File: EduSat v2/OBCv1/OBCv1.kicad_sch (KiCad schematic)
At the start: 10 parts, among them J1 Conn_02x20_Odd_Even, J2 USB_C_Receptacle_USB2.0_16P, U1 ESP32-WROOM-32E, U2 CP2102N-Axx-xQFN28, U3 Ai-Thinker-Ra-02

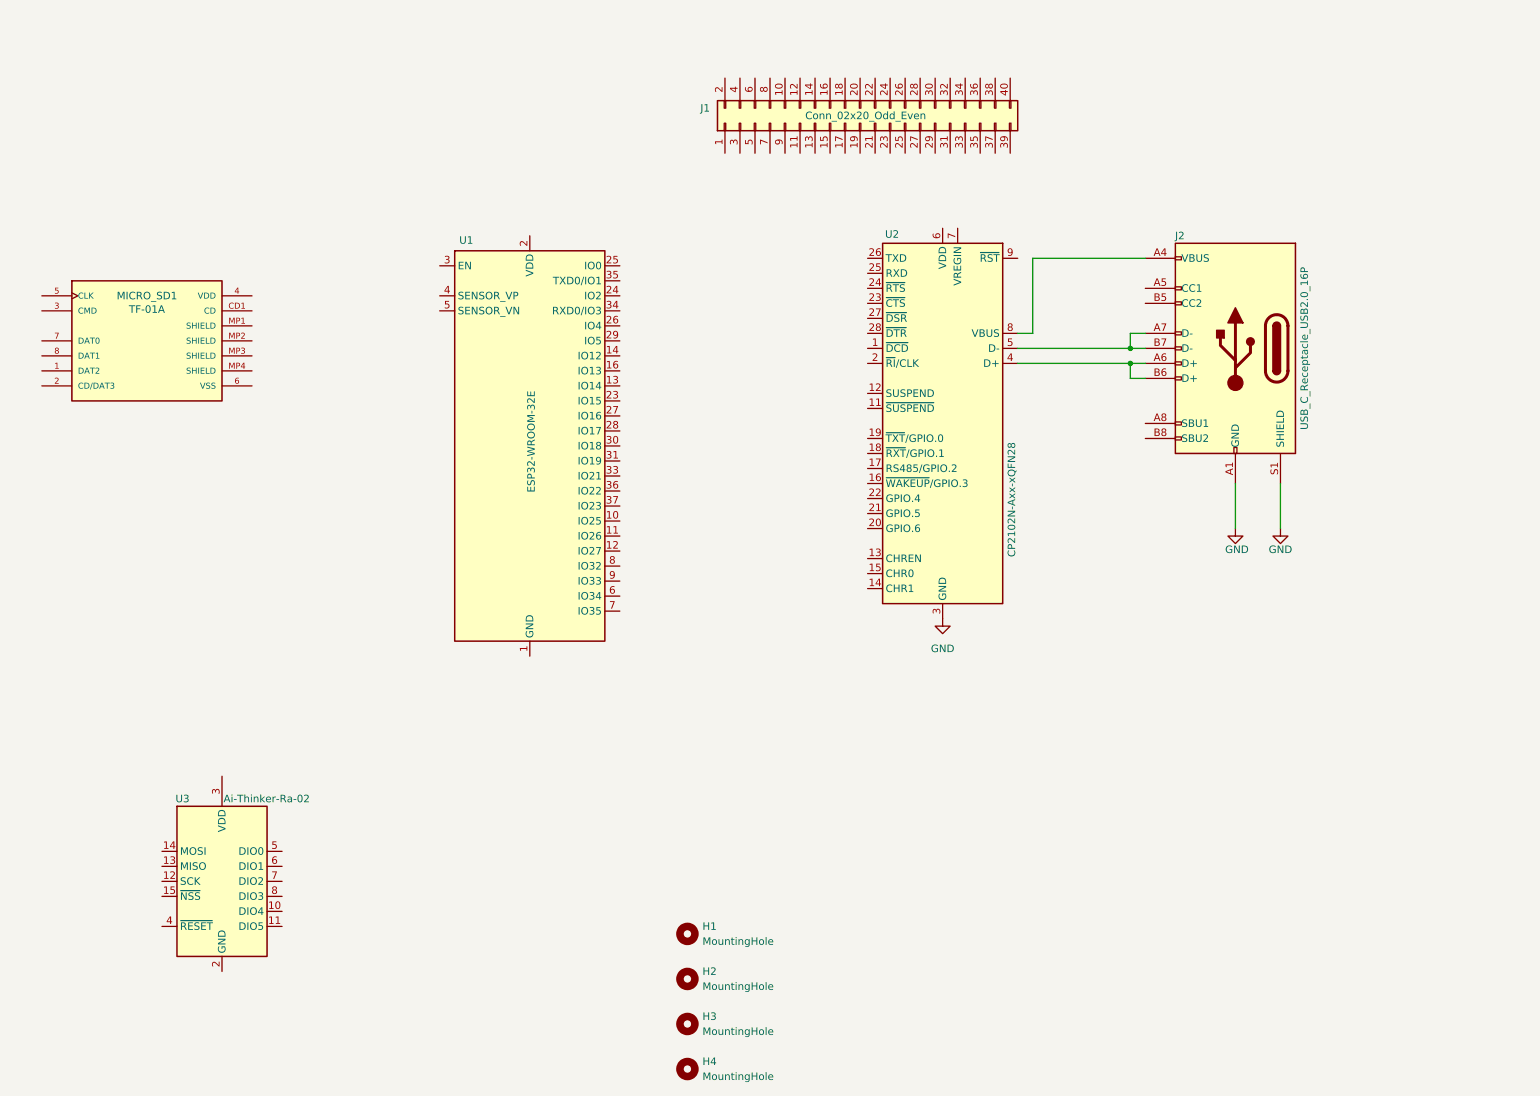
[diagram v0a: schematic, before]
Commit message: a
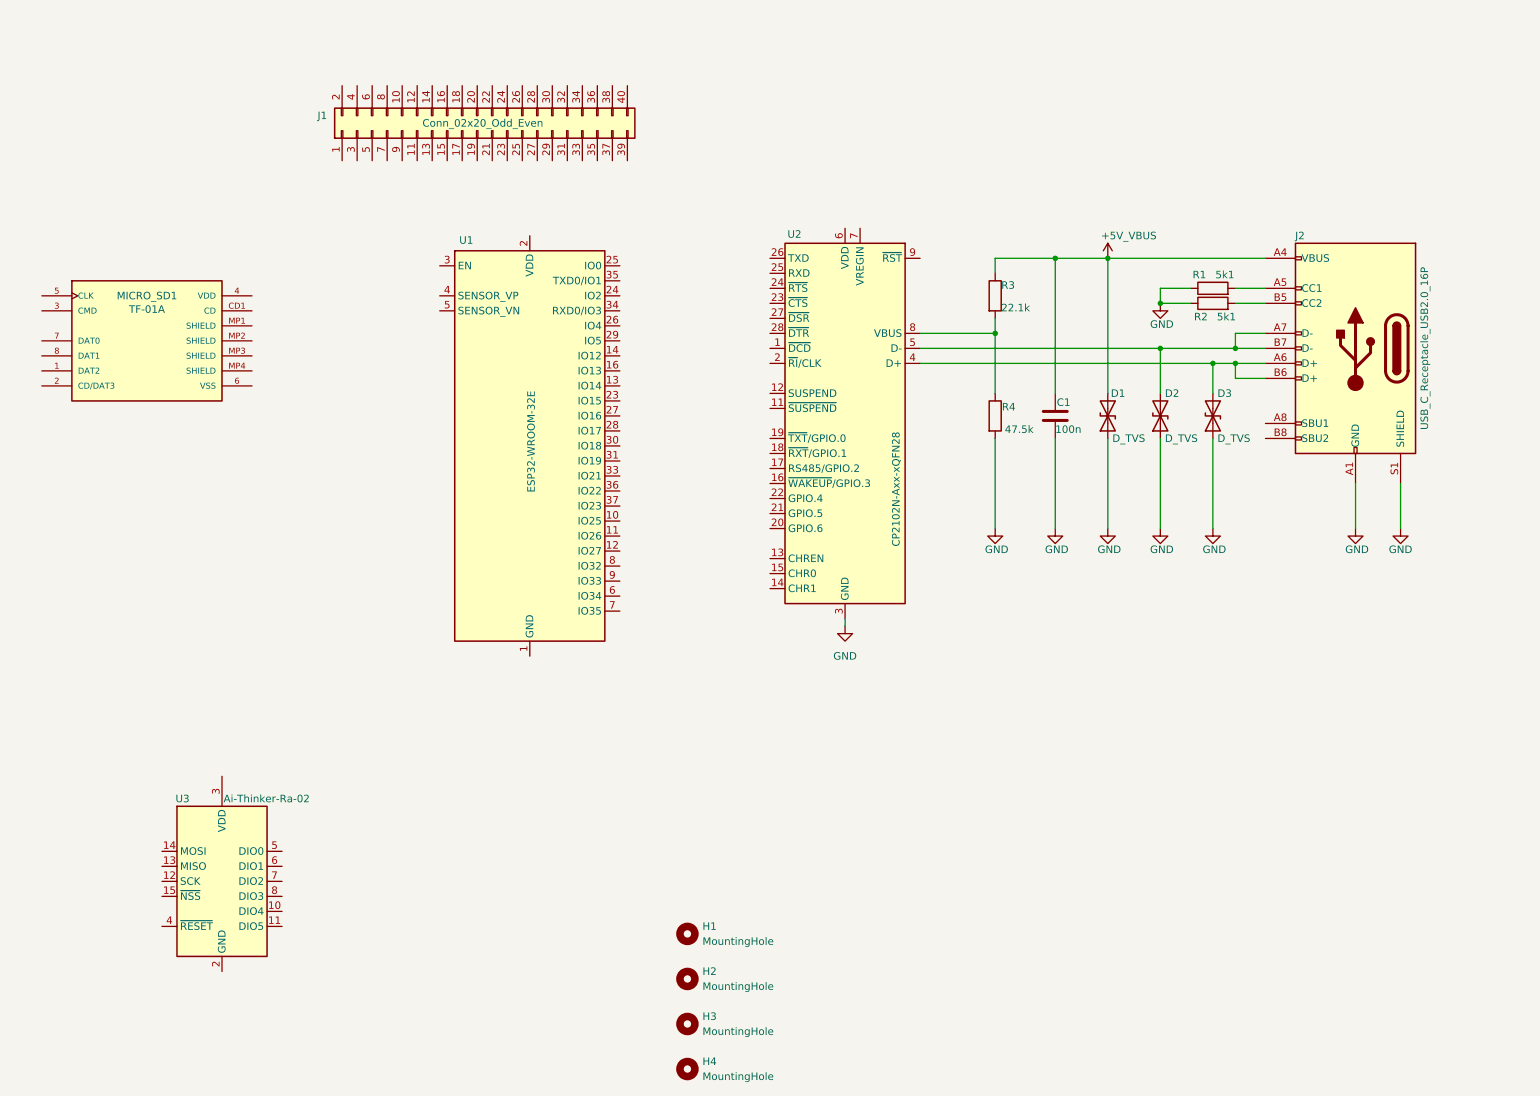
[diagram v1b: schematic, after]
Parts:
- added C1: 100n, Capacitor_SMD:C_0805_2012Metric, symbol Device:C
- added D1, D2, D3: D_TVS, Diode_SMD:D_0603_1608Metric, symbol Device:D_TVS
- added R1, R2: 5k1, Resistor_SMD:R_0805_2012Metric, symbol Device:R
- added R3: 22.1k, symbol Device:R
- added R4: 47.5k, symbol Device:R
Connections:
- net GND: now also C1.2, D1.1 (A1), D2.1 (A1), D3.1 (A1), R1.1, R2.1, R4.2
- net +5V_VBUS: now reaches J2.A4 (VBUS), J2.A9 (VBUS), J2.B4 (VBUS), J2.B9 (VBUS)
- net +5V_VBUS: now also C1.1, D1.2 (A2), R3.1; no longer U2.8 (VBUS)
- net at J2.A5 (CC1): now also R1.2
- net at J2.A6 (D+), J2.B6 (D+), U2.4 (D+): now also D3.2 (A2)
- net at J2.A7 (D-), J2.B7 (D-), U2.5 (D-): now also D2.2 (A2)
- net at J2.B5 (CC2): now also R2.2
- new net: R3.2, R4.1, U2.8 (VBUS)
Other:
- moved on the sheet: J1, J2, U2

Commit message: Updates
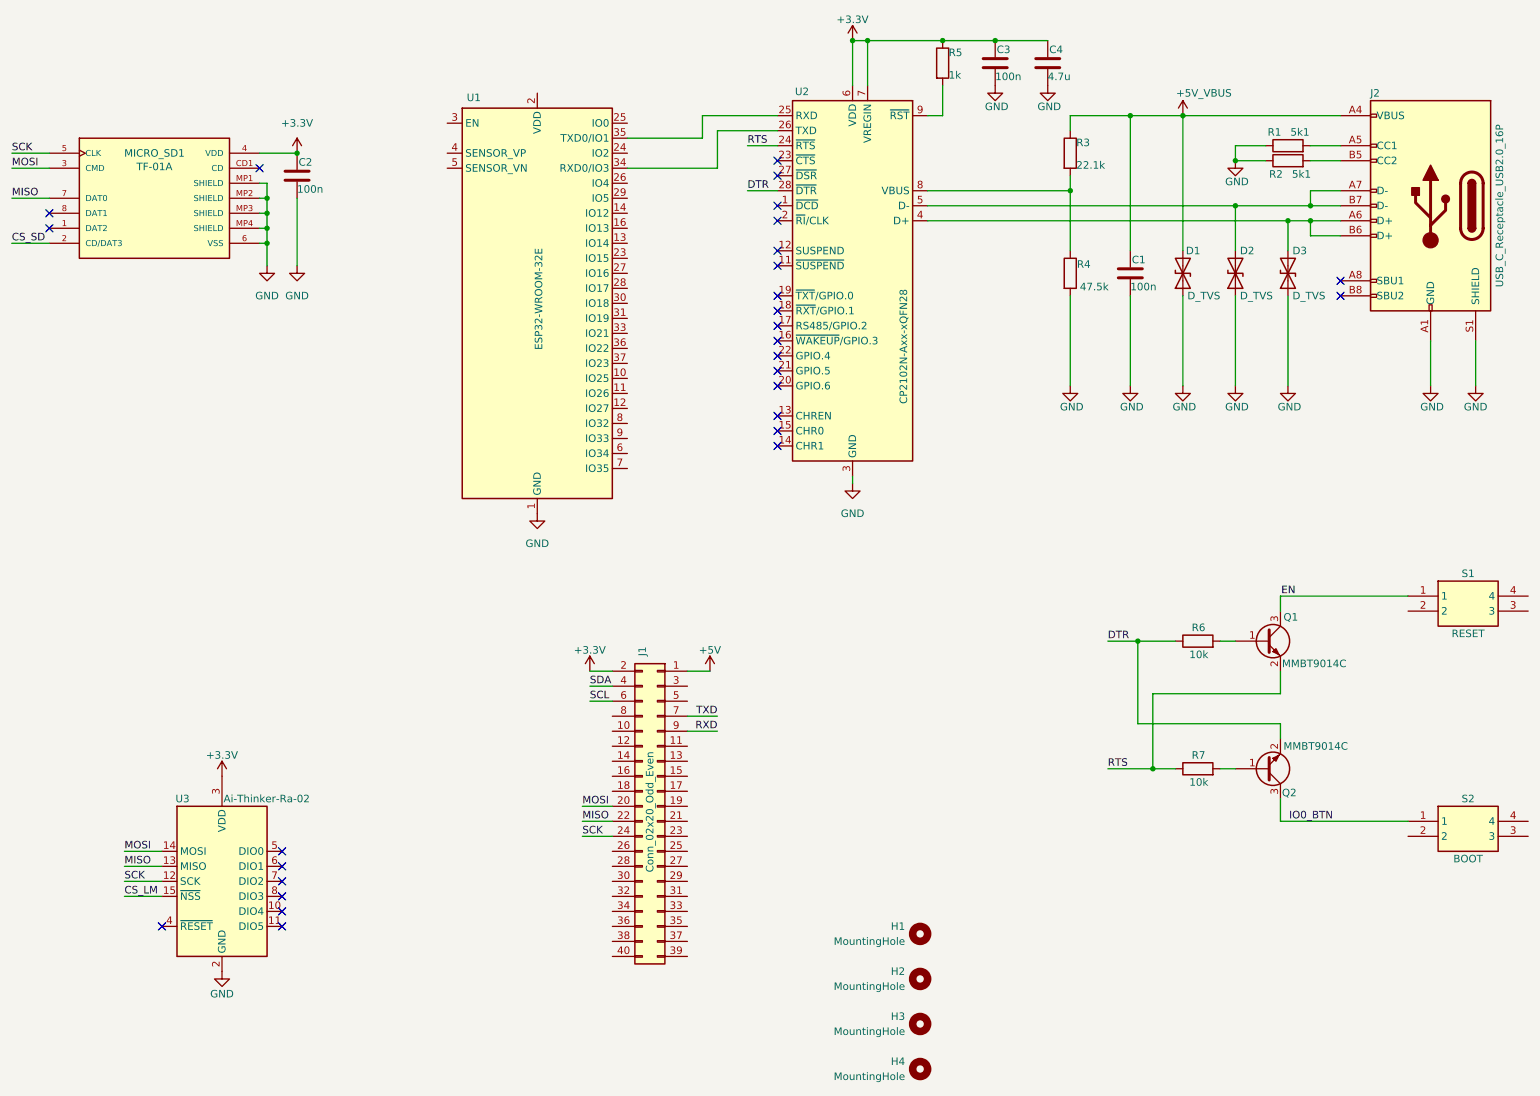
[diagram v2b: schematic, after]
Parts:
- added C2, C3: 100n, Capacitor_SMD:C_0805_2012Metric, symbol Device:C
- added C4: 4.7u, Capacitor_SMD:C_0805_2012Metric, symbol Device:C
- added Q1, Q2: MMBT9014C, Package_TO_SOT_SMD:SOT-23, symbol Transistor_BJT:BC848
- added R5: 1k, symbol Device:R
- added R6, R7: 10k, symbol Device:R
- added S1: RESET, PTS647SM50SMTR2LFS, symbol PTS647SM50SMTR2LFS:PTS647SM50SMTR2LFS
- added S2: BOOT, PTS647SM50SMTR2LFS, symbol PTS647SM50SMTR2LFS:PTS647SM50SMTR2LFS
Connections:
- net GND: now also MICRO_SD1.6 (VSS), MICRO_SD1.MP1 (SHIELD), MICRO_SD1.MP2 (SHIELD), MICRO_SD1.MP3 (SHIELD), MICRO_SD1.MP4 (SHIELD), U1.1 (GND), U1.15 (GND), U1.38 (GND), U1.39 (GND), U3.1 (GND), U3.16 (GND), U3.2 (GND), U3.9 (GND), C2.2, C3.2, C4.2
- net CS_SD: now reaches MICRO_SD1.2 (CD/DAT3)
- net MOSI: now reaches MICRO_SD1.3 (CMD)
- net MOSI: now also J1.20 (Pin_20), U3.14 (MOSI)
- net +3.3V: now reaches MICRO_SD1.4 (VDD)
- net +3.3V: now also J1.2 (Pin_2), U2.6 (VDD), U2.7 (VREGIN), U3.3 (VDD), C2.1, C3.1, C4.1, R5.1
- net SCK: now reaches MICRO_SD1.5 (CLK)
- net SCK: now also J1.24 (Pin_24), U3.12 (SCK)
- net MISO: now reaches MICRO_SD1.7 (DAT0)
- net MISO: now also J1.22 (Pin_22), U3.13 (MISO)
- net +5V: now reaches J1.1 (Pin_1)
- net SDA: now reaches J1.4 (Pin_4)
- net SCL: now reaches J1.6 (Pin_6)
- net TXD: now reaches J1.7 (Pin_7)
- net RXD: now reaches J1.9 (Pin_9)
- net RTS: now reaches U2.24 (~{RTS})
- net RTS: now also Q1.2 (E), R7.1
- net at U2.25 (RXD): now also U1.35 (TXD0/IO1)
- net at U2.26 (TXD): now also U1.34 (RXD0/IO3)
- net DTR: now reaches U2.28 (~{DTR})
- net DTR: now also Q2.2 (E), R6.1
- net at U2.9 (~{RST}): now also R5.2
- net CS_LM: now reaches U3.15 (~{NSS})
- new net: Q2.1 (B), R7.2
- new net: Q1.1 (B), R6.2
- new net EN: Q1.3 (C), S1.1
- new net IO0_BTN: Q2.3 (C), S2.1
- no-connect marks 0 -> 28
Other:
- moved on the sheet: C1, D1, D2, D3, H1, H2, H3, H4, J1, J2, MICRO_SD1, R1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
